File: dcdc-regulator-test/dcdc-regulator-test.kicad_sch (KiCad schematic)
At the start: 8 parts, among them U1 AP63205WU, U2 MIC5504-3.3YM5

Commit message: example layout
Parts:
- U2: footprint Package_TO_SOT_SMD:SOT-23-5_HandSoldering -> Package_TO_SOT_SMD:SOT-23-5
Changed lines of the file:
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@@
 			)
 		)
-		(property "Footprint" "Package_TO_SOT_SMD:SOT-23-5_HandSoldering"
+		(property "Footprint" "Package_TO_SOT_SMD:SOT-23-5"
 			(at 184.15 67.31 0)
 			(effects

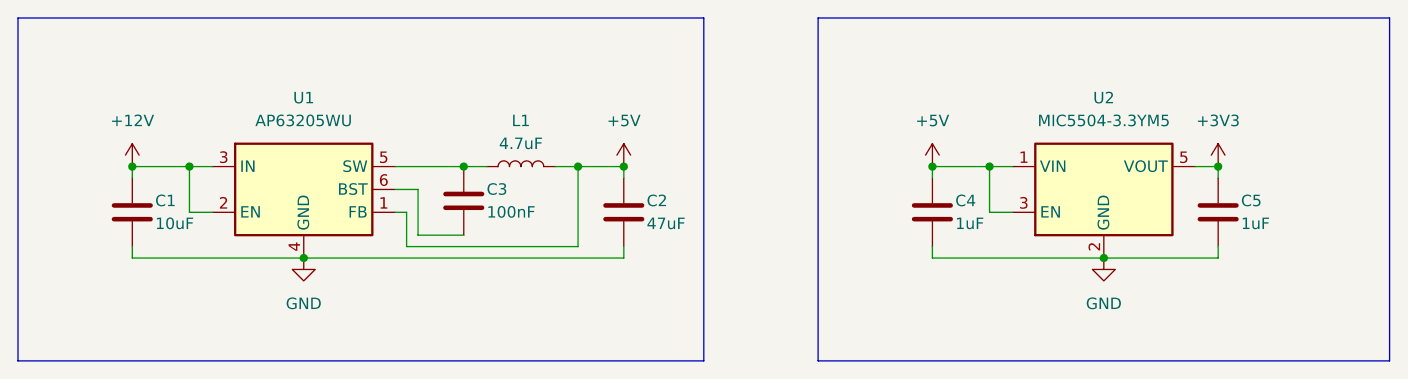
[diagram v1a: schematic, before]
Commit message: Added power regulators to design blocks library
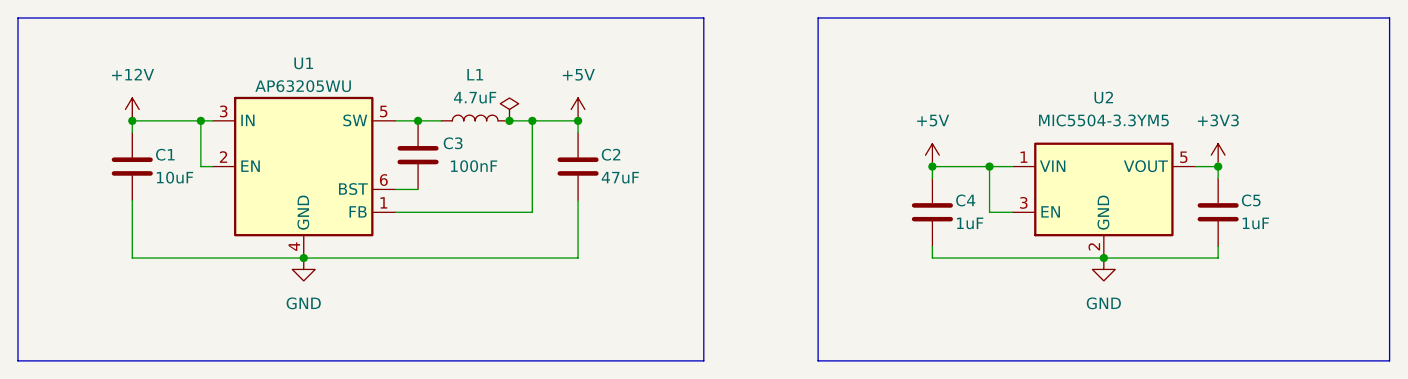
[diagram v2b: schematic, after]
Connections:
- net at L1.1, U1.5 (SW): now also C3.1; no longer C3.2
- net at U1.6 (BST): now also C3.2; no longer C3.1
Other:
- moved on the sheet: C1, C2, C3, L1, U1
